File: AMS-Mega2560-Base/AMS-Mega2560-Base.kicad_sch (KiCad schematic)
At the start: 29 parts, among them J1 Conn_01x03, J2 Conn_01x03, J3 Conn_01x08, J4 Sense1, J5 Sense2, J6 AdafruitUltimateGPS, J7 Conn_02x03_Odd_Even, J8 Conn_01x03, P1 Power, P10 CONN_01X01, P11 CONN_01X01, P12 CONN_01X01, P13 CONN_01X01, P2 Analog, P3 Analog, P4 Digital, P5 PWM, P6 PWM, P7 Communication, P8 CONN_01X01, P9 CONN_01X01, T1 Conn_01x08, T2 Conn_01x08, T3 Conn_01x08, T4 Conn_01x08, T5 Conn_01x08, T6 Conn_01x08

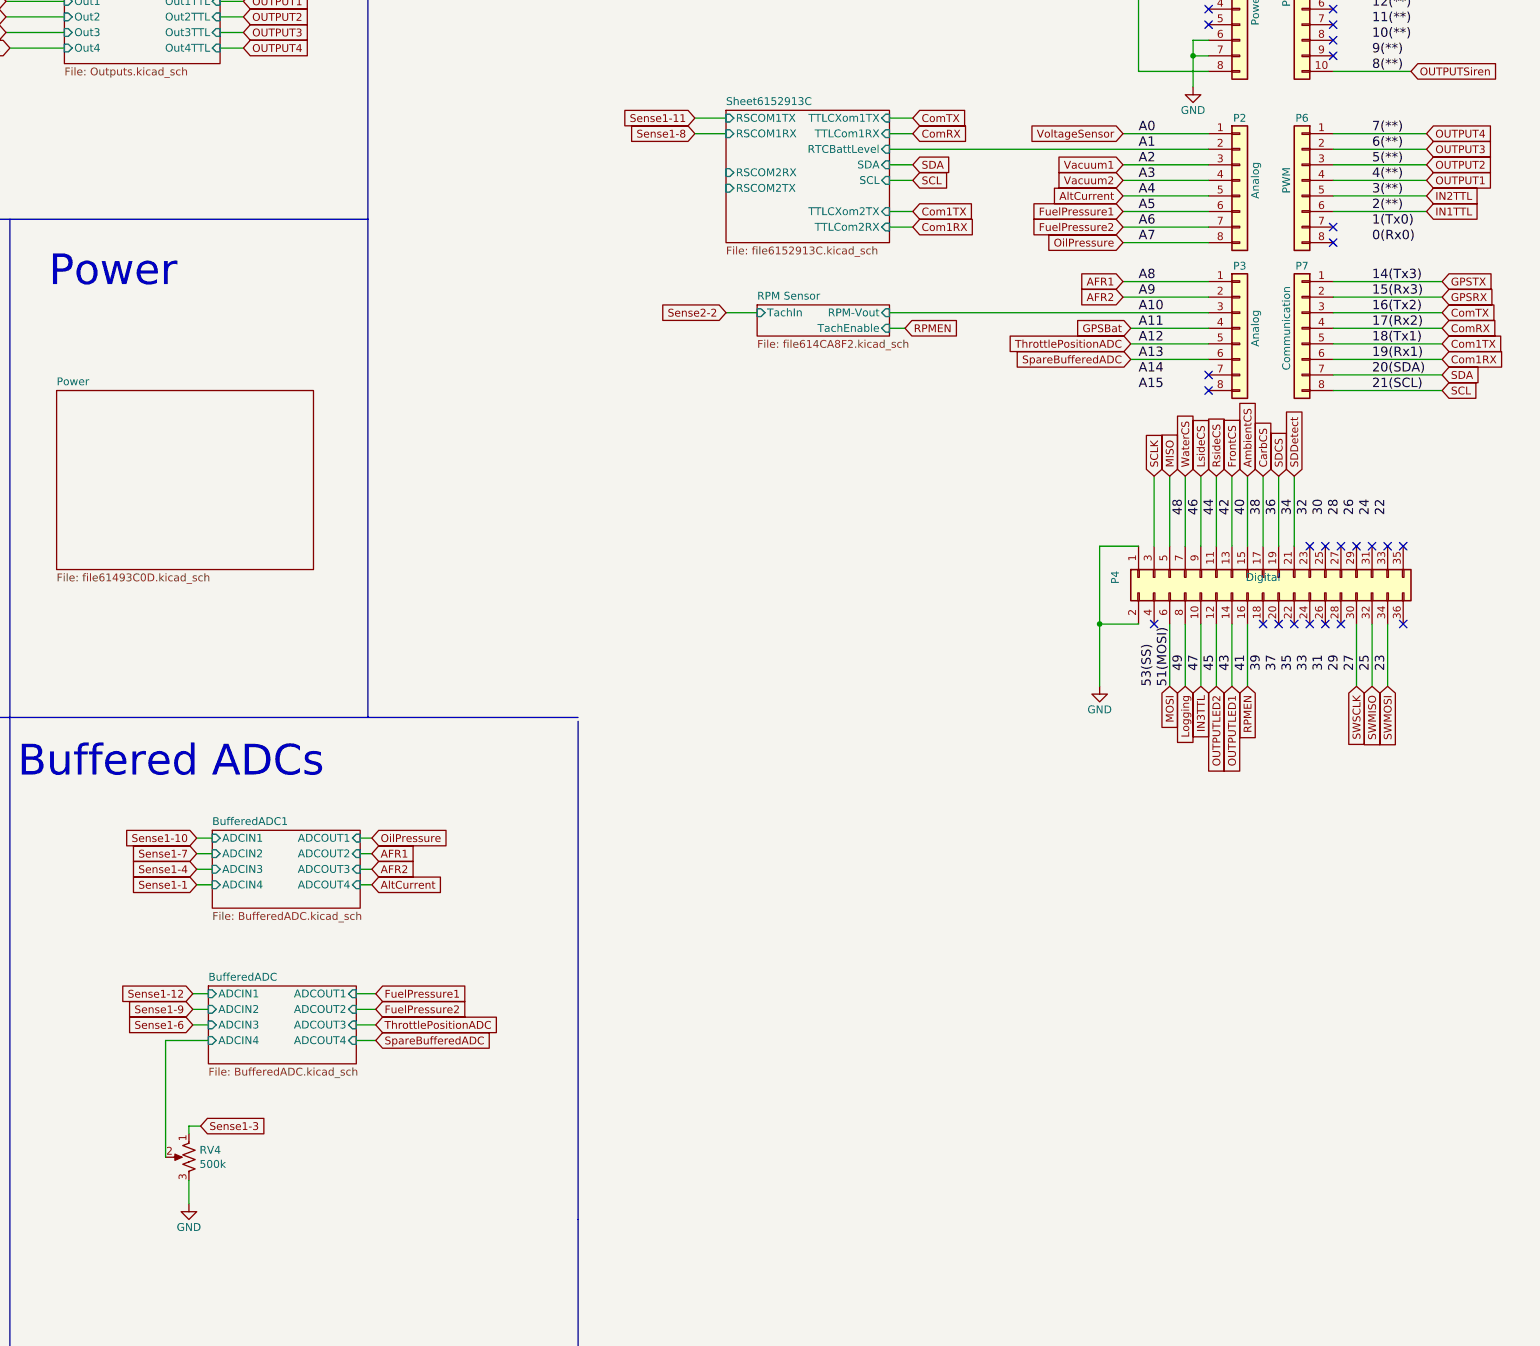
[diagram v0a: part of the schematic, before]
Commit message: updating this for the merge.
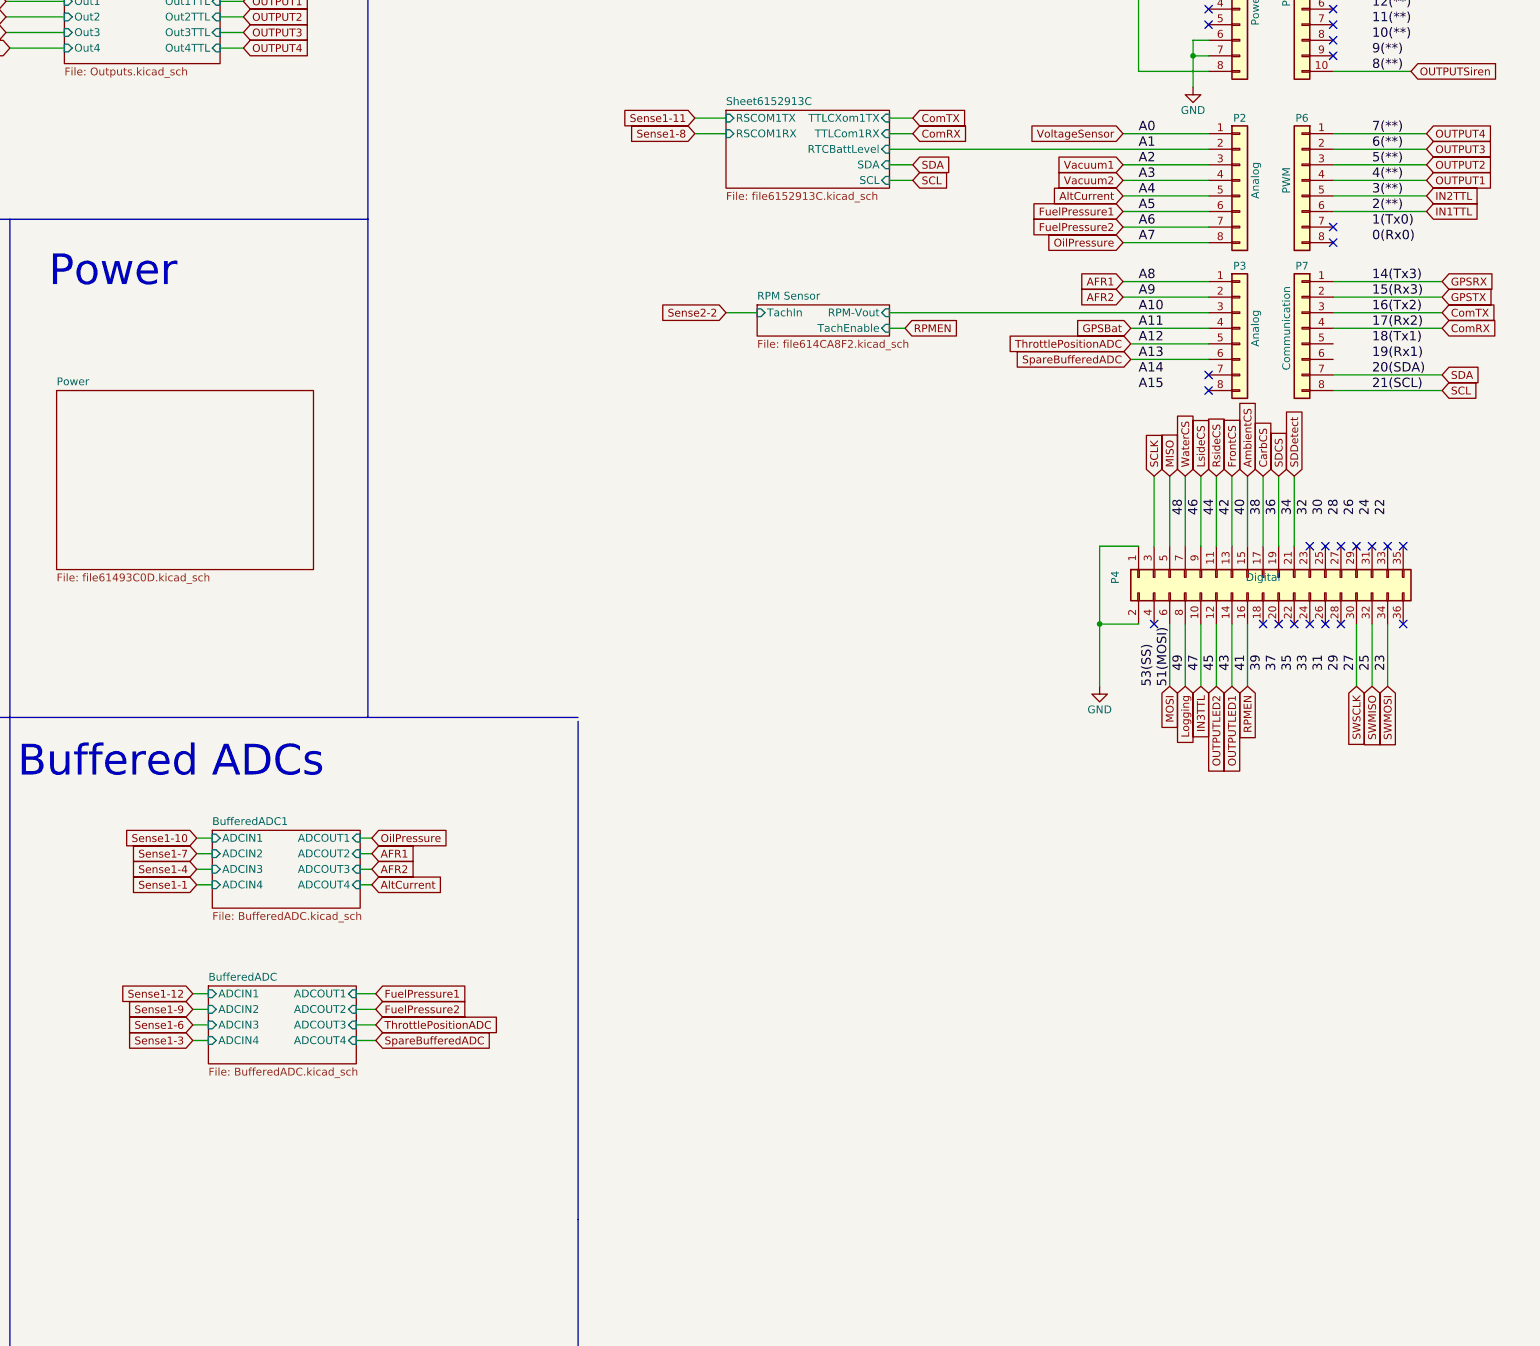
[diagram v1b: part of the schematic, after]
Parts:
- removed RV4: 500k, Potentiometer_THT:Potentiometer_Bourns_3296W_Vertical, symbol Device:R_POT_US
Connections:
- net GPSRX: now also P7.1 (Pin_1); no longer P7.2 (Pin_2)
- net GPSTX: now also P7.2 (Pin_2); no longer P7.1 (Pin_1)
- net Com1RX: no longer names the net of P7.6 (Pin_6)
- net Com1TX: no longer names the net of P7.5 (Pin_5)
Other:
- sheet Sheet6152913C ports: added none; removed RSCOM2RX, RSCOM2TX, TTLCXom2TX, TTLCom2RX
